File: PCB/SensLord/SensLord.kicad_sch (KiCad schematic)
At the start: 26 parts, among them J111 USB_B_Micro, Q120 IRLML6402, U1 ESP32-C6-MINI-1, U110 MCP73831-2-OT, U140 MCP1700x-330xxTT

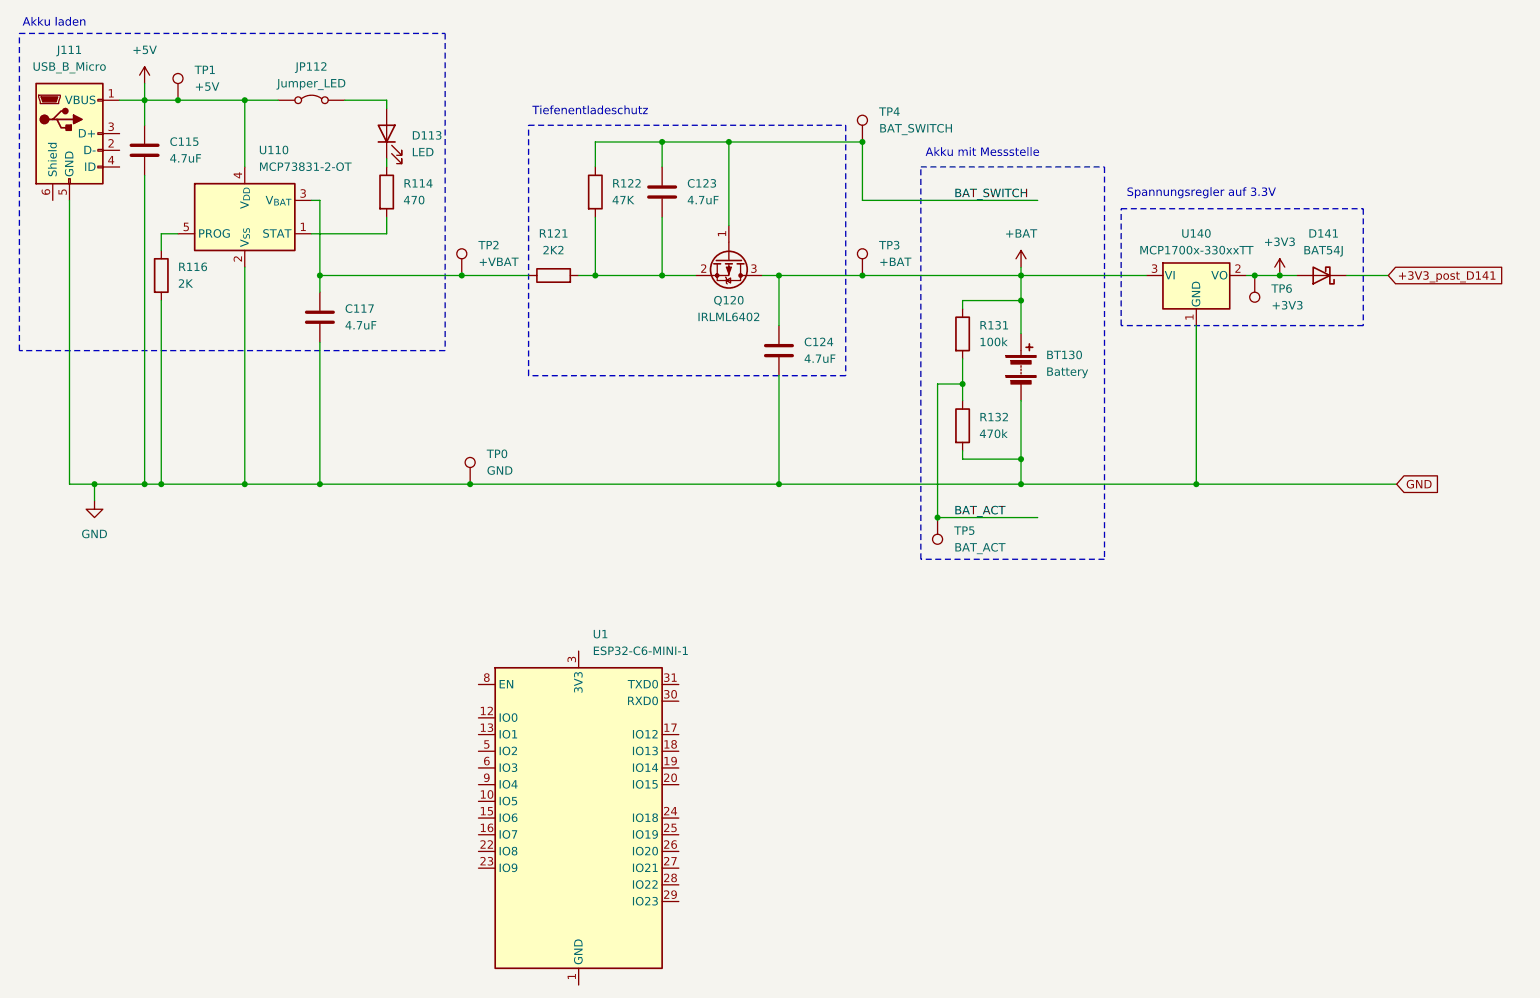
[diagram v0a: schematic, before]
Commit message: testing circuit ..
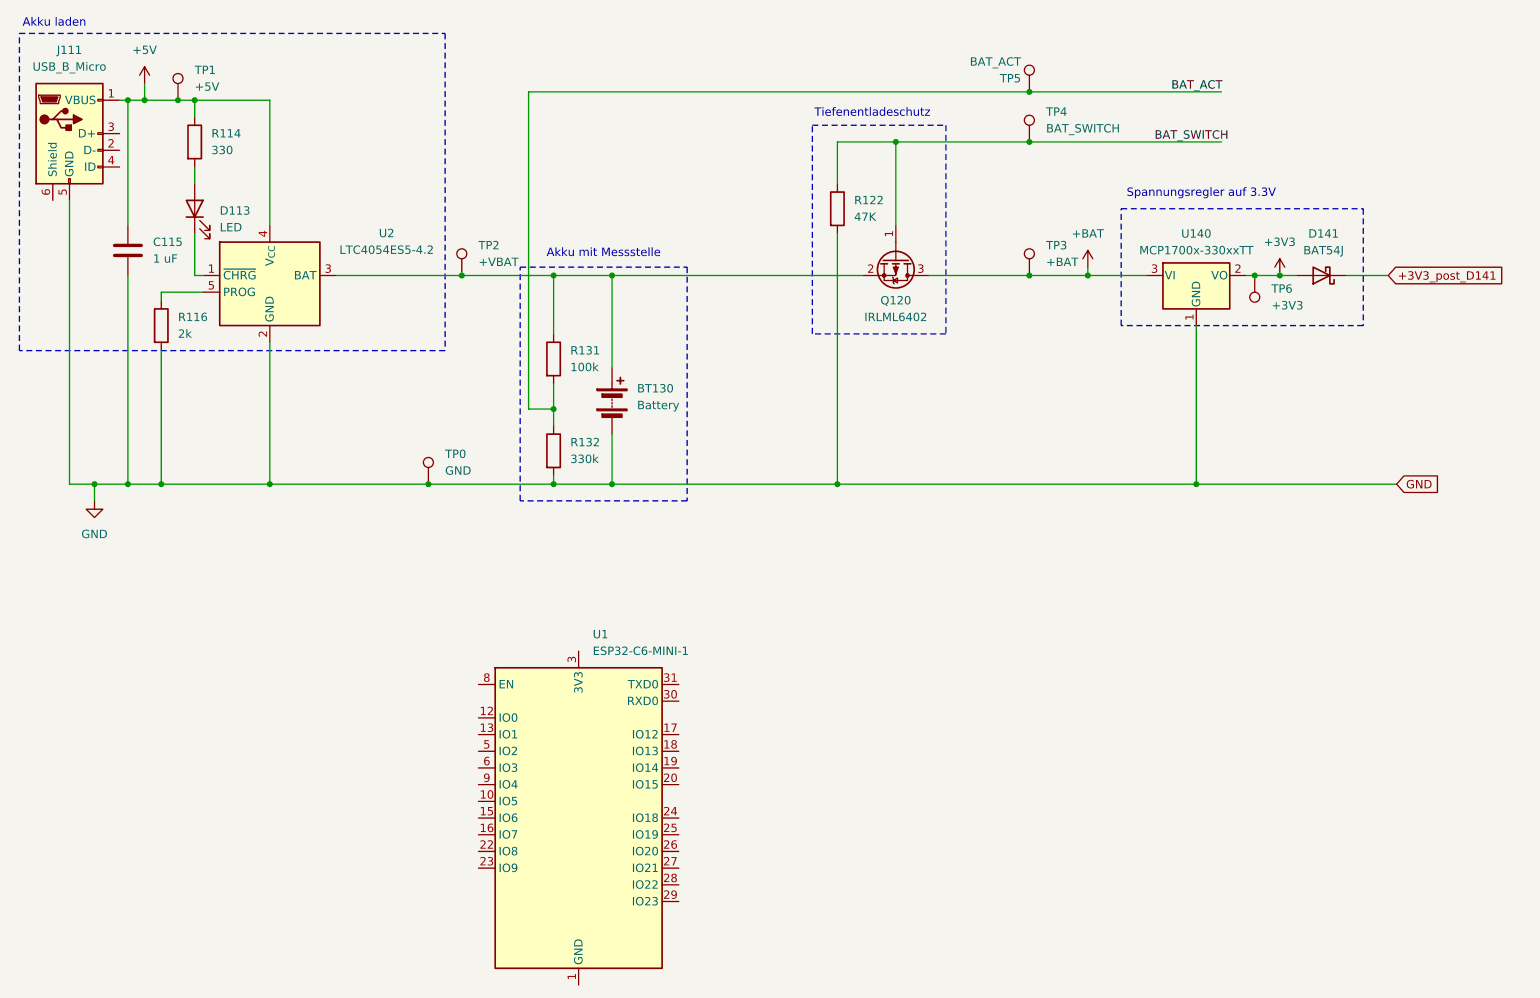
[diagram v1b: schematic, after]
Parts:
- removed C117, C123, C124: 4.7uF, Capacitor_SMD:C_1206_3216Metric, symbol Device:C
- removed JP112: Jumper_LED, Connector_PinHeader_2.54mm:PinHeader_2x02_P2.54mm_Vertical_SMD, symbol Jumper:Jumper_2_Bridged
- removed R121: 2K2, Resistor_SMD:R_0603_1608Metric, symbol Device:R
- removed U110: MCP73831-2-OT, Package_TO_SOT_SMD:SOT-23-5, symbol Battery_Management:MCP73831-2-OT
- added U2: LTC4054ES5-4.2, Package_TO_SOT_SMD:TSOT-23-5, symbol Battery_Management:LTC4054ES5-4.2
- C115: value 4.7uF -> 1 uF
- R114: value 470 -> 330
- R116: value 2K -> 2k
- R132: value 470k -> 330k
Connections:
- net +5V: now also R114.1, U2.4 (V_{CC})
- net +BAT: no longer BT130.1 (+), R131.1
- net GND: now also R122.2, U2.2 (GND)
- net at Q120.2 (S): now also BT130.1 (+), R131.1, TP2.1, U2.3 (BAT); no longer R122.2
- net at D113.1 (K): now also U2.1 (~{CHRG}); no longer R114.1
- net at D113.2 (A): now also R114.2
- net at R116.1: now also U2.5 (PROG)
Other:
- moved on the sheet: BT130, C115, D113, Q120, R114, R116, R122, R131, R132, TP0, TP3, TP4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
